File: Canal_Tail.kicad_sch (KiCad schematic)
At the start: 0 parts

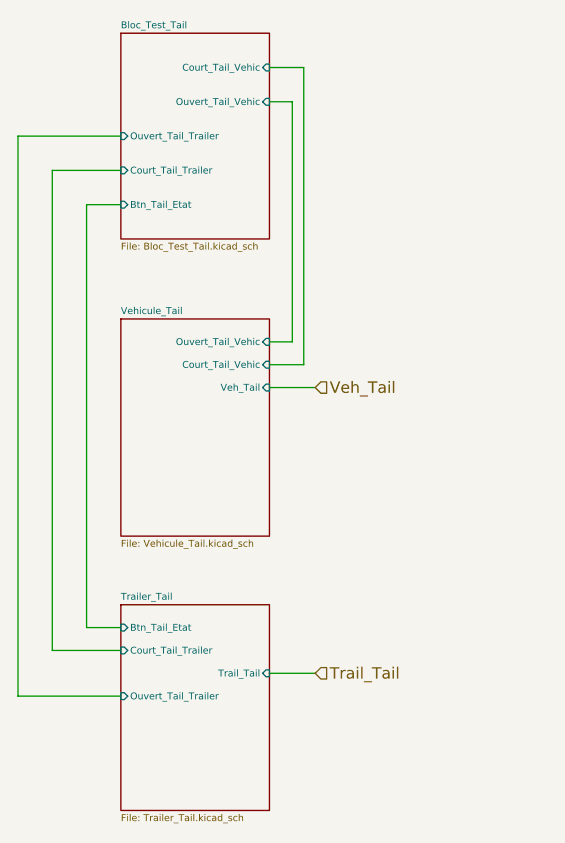
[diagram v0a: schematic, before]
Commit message: Add files via upload
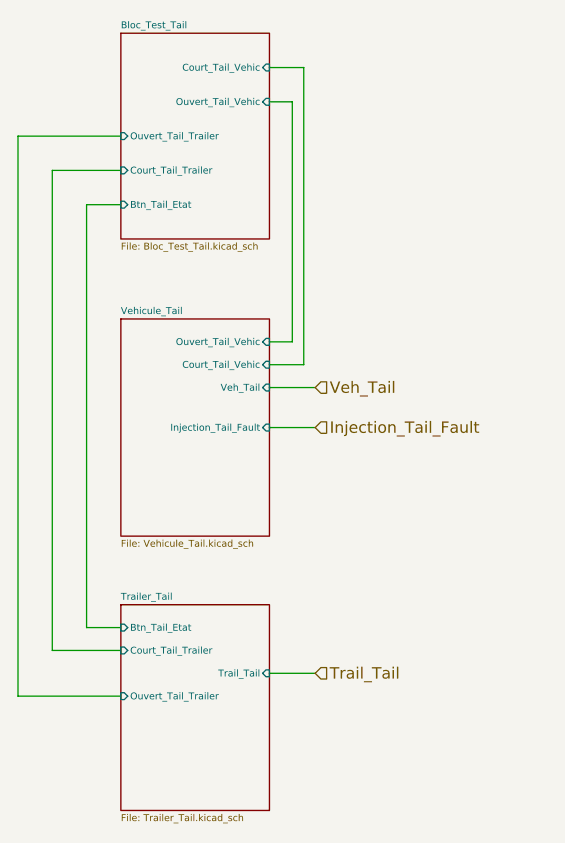
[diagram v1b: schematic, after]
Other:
- sheet Vehicule_Tail ports: added Injection_Tail_Fault; removed none
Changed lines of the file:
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@@
+	(wire
+		(pts
+			(xy 59.69 60.325) (xy 64.77 60.325)
+		)
+		(stroke
+			(width 0)
+			(type default)
+		)
+	)
 	(wire
 		(pts
@@
 			(width 0)
 			(type default)
+		)
+	)
+	(hierarchical_label "Injection_Tail_Fault"
+		(shape input)
+		(at 64.77 60.325 0)
+		(effects
+			(font
+				(size 1.27 1.27)
+			)
+			(justify left)
 		)
 	)
@@
 			(effects
 				(font
+					(size 0.762 0.762)
+				)
+				(justify right)
+			)
+		)
+		(pin "Injection_Tail_Fault" input
+			(at 59.69 60.325 0)
+			(effects
+				(font

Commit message: Add files via upload
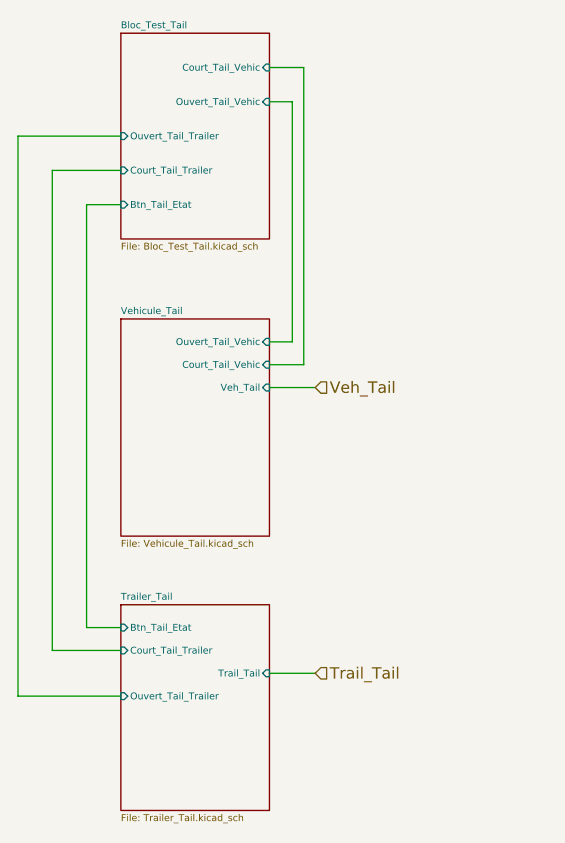
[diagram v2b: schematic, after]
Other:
- sheet Vehicule_Tail ports: added none; removed Injection_Tail_Fault
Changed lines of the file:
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@@
-	(wire
-		(pts
-			(xy 59.69 60.325) (xy 64.77 60.325)
-		)
-		(stroke
-			(width 0)
-			(type default)
-		)
-	)
 	(wire
 		(pts
@@
 			(width 0)
 			(type default)
-		)
-	)
-	(hierarchical_label "Injection_Tail_Fault"
-		(shape input)
-		(at 64.77 60.325 0)
-		(effects
-			(font
-				(size 1.27 1.27)
-			)
-			(justify left)
 		)
 	)
@@
 			(effects
 				(font
-					(size 0.762 0.762)
-				)
-				(justify right)
-			)
-		)
-		(pin "Injection_Tail_Fault" input
-			(at 59.69 60.325 0)
-			(effects
-				(font
